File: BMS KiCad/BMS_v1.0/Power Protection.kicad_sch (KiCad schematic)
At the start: 19 parts, among them J1 Conn_01x02, J2 Conn_01x02, Q1 PMOS, Q2 PMOS, Q3 NMOS, Q4 NMOS

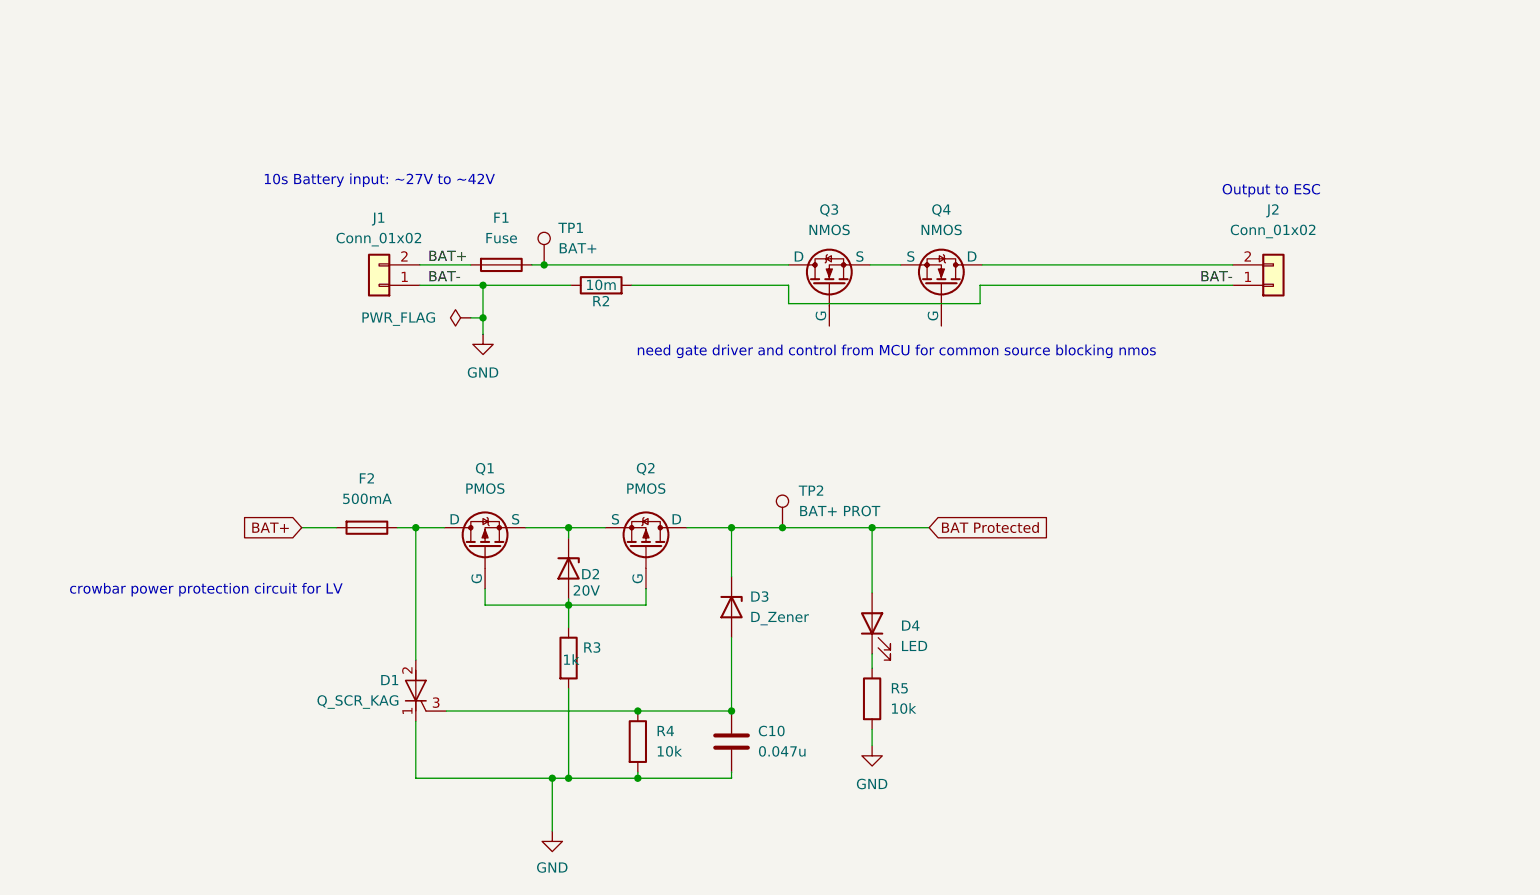
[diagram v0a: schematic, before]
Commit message: TI IC done except for I2C and precharge circuit
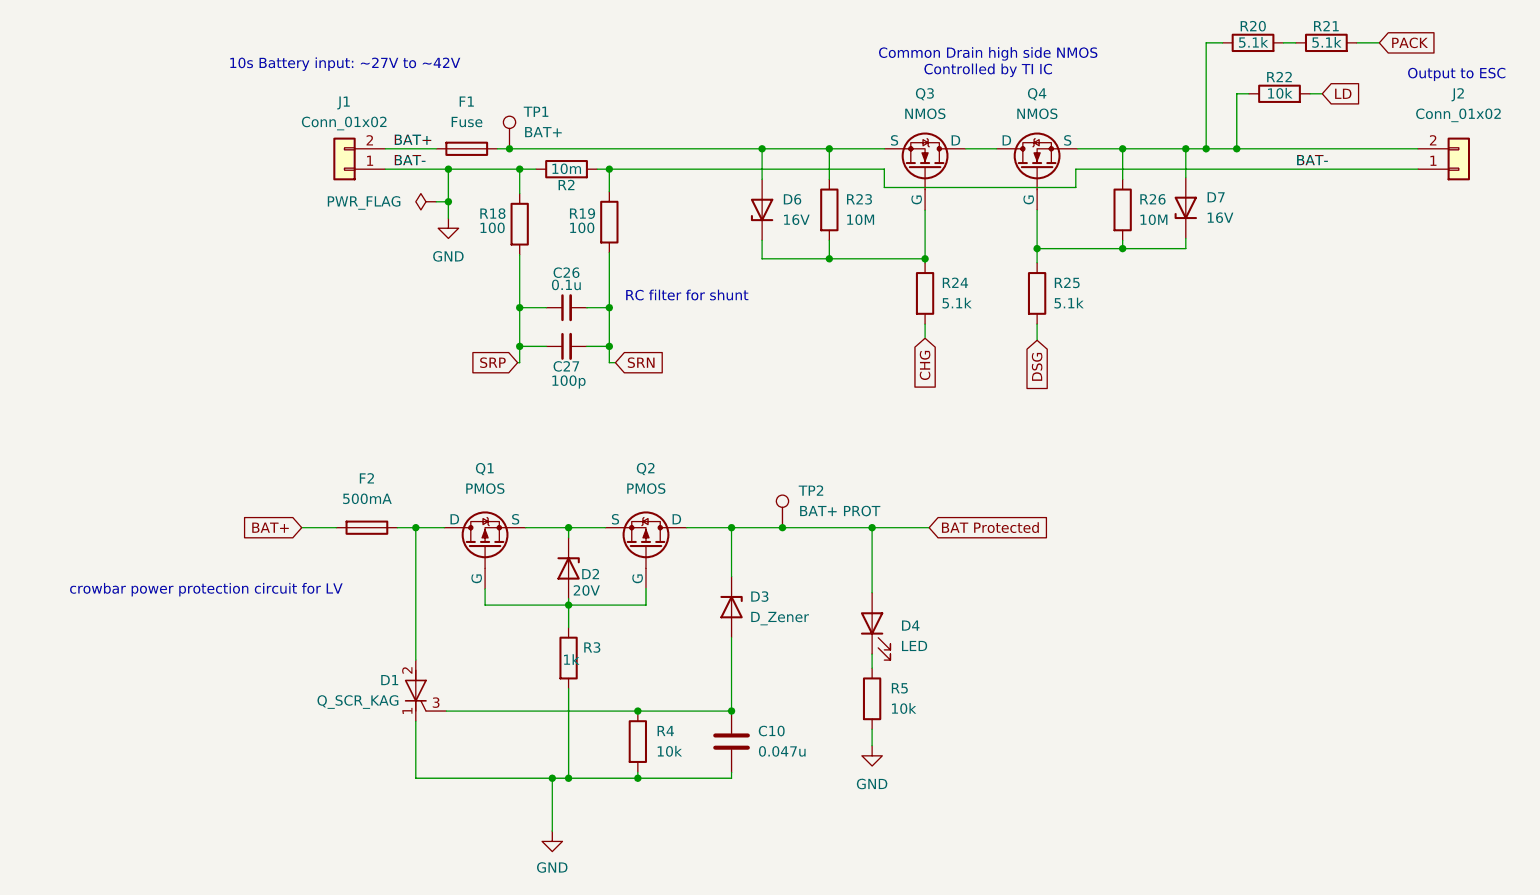
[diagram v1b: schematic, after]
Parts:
- added C26: 0.1u, symbol Device:C_Small
- added C27: 100p, symbol Device:C_Small
- added D6, D7: 16V, symbol Device:D_Zener
- added R18, R19: 100, symbol Device:R
- added R20, R21, R24, R25: 5.1k, symbol Device:R
- added R22: 10k, symbol Device:R
- added R23, R26: 10M, symbol Device:R
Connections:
- net GND: now also R18.1, R19.1
- net at F1.1, TP1.1: now also Q3.3 (S), D6.2 (A), R23.1; no longer Q3.1 (D)
- net at Q3.2 (G): now also D6.1 (K), R23.2, R24.1
- net at Q4.3 (S): now also J2.2 (Pin_2), D7.2 (A), R20.1, R22.1, R26.1; no longer Q3.3 (S)
- net at Q4.1 (D): now also Q3.1 (D); no longer J2.2 (Pin_2)
- net at Q4.2 (G): now also D7.1 (K), R25.1, R26.2
- new net: R20.2, R21.1
- new net CHG: R24.2
- new net DSG: R25.2
- new net LD: R22.2
- new net PACK: R21.2
- new net SRN: C26.2, C27.2, R19.2
- new net SRP: C26.1, C27.1, R18.2
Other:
- note added: "Common Drain high side NMOS Controlled by TI IC"
- note added: "RC filter for shunt"
- note removed: "need gate driver and control from MCU for common source blocking nmos"
- moved on the sheet: F1, J1, J2, Q3, Q4, R2, TP1
